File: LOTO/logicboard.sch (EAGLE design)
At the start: 31 parts, among them IC1 74ALS08N, IC2 74ALS08N, Q1 BSS92, Q2 BSS101

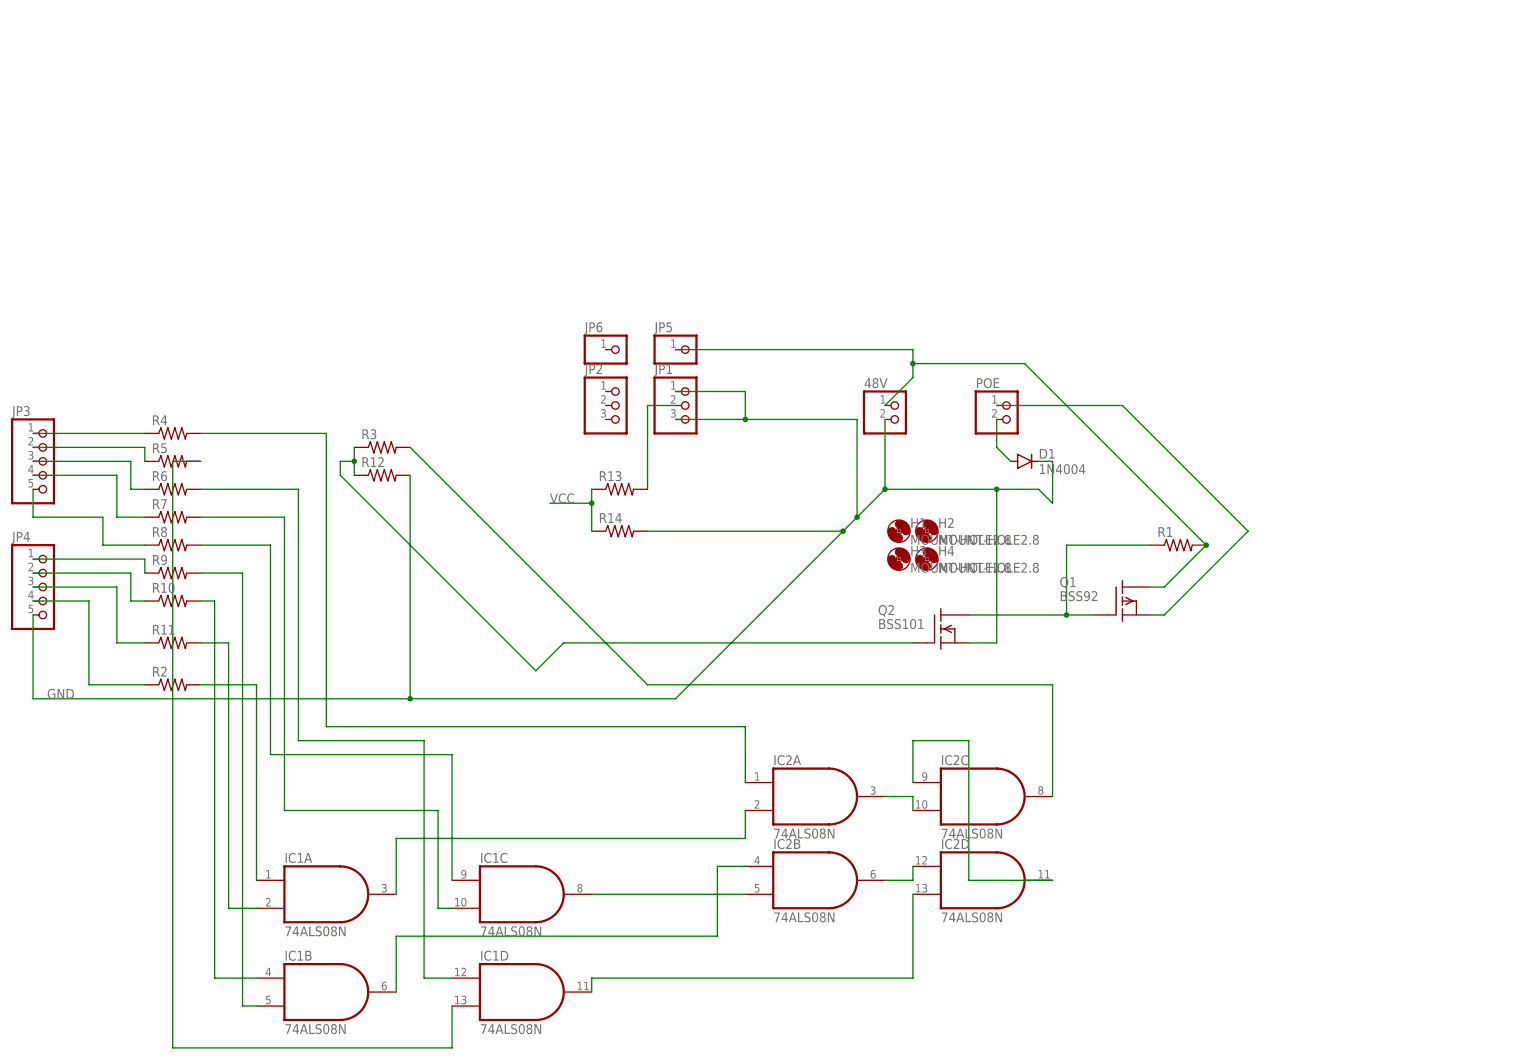
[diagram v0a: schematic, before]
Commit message: route management
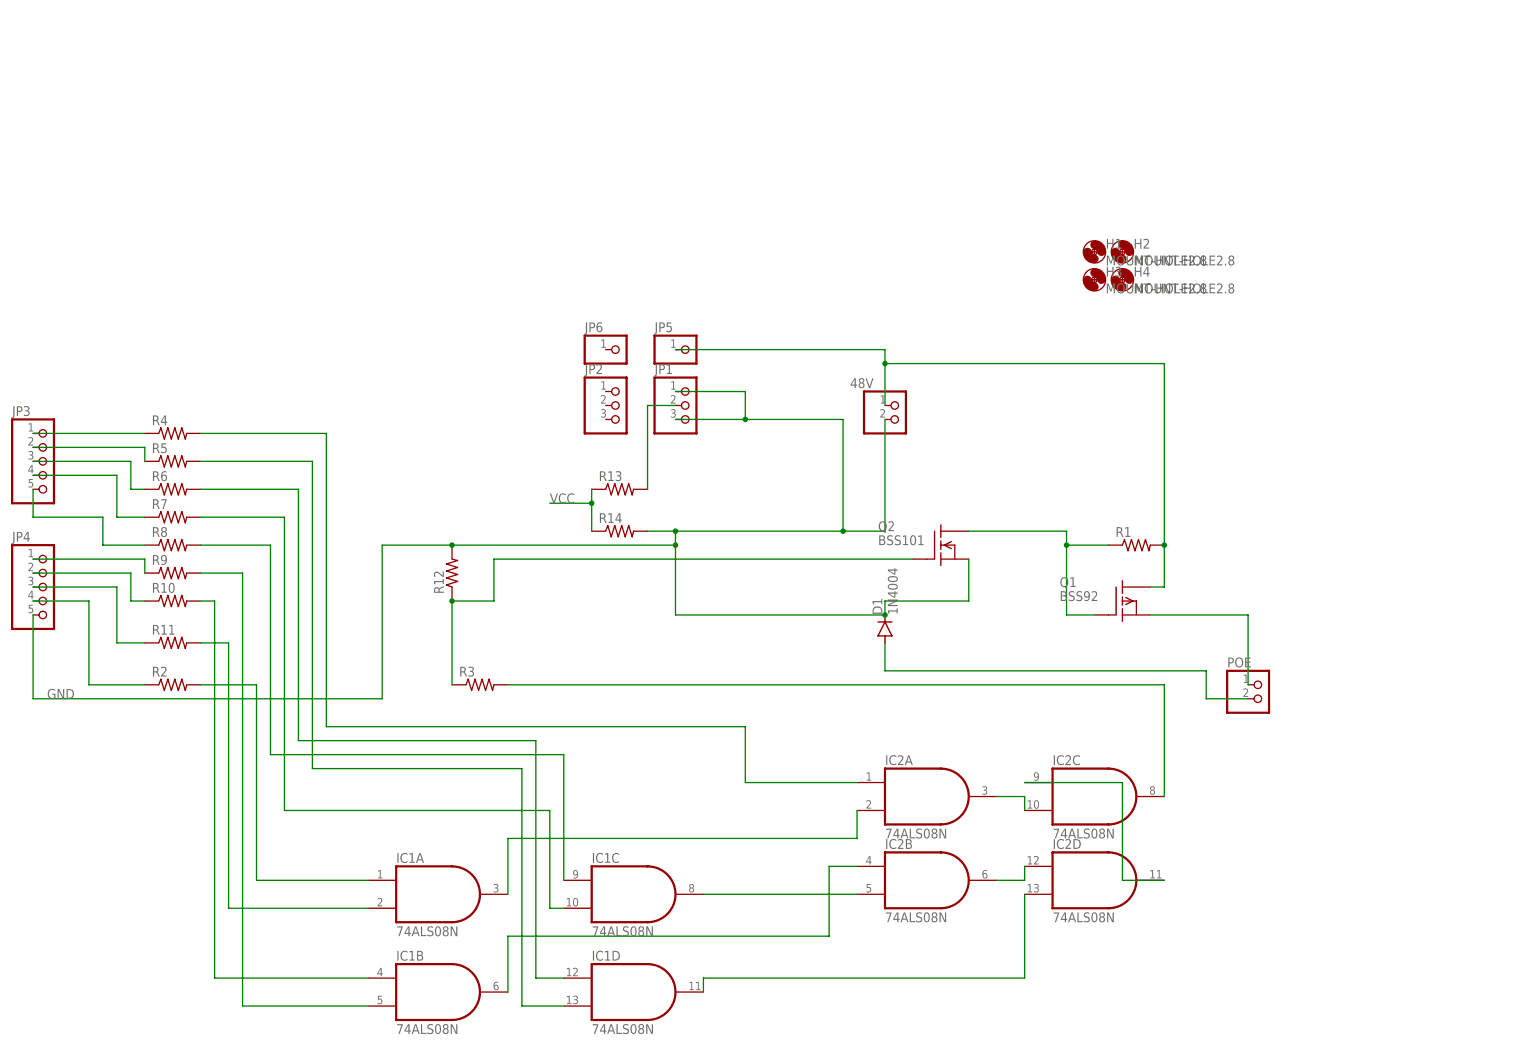
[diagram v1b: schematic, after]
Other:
- moved on the sheet: D1, H1, H2, H3, H4, IC1A, IC1B, IC1C, IC1D, IC2A, IC2B, IC2C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

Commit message: reduced AC board size, attributes, bom
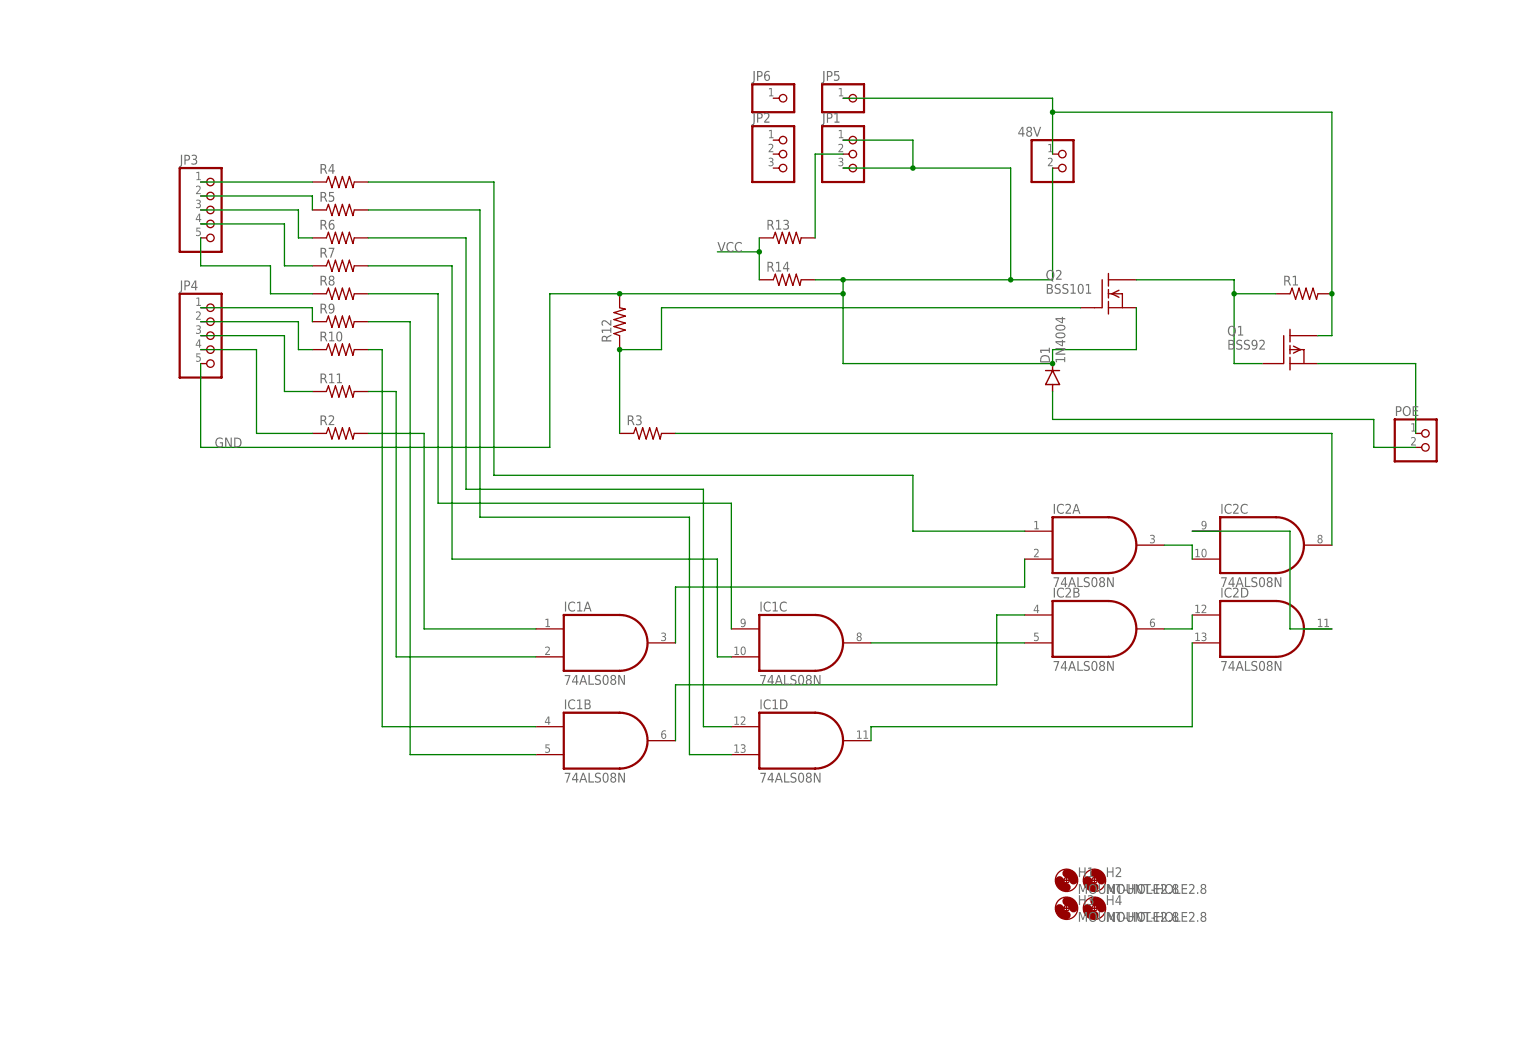
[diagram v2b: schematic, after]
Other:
- moved on the sheet: 48V, D1, H1, H2, H3, H4, IC1A, IC1B, IC1C, IC1D, IC2A, IC2B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

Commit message: added attributes to loto
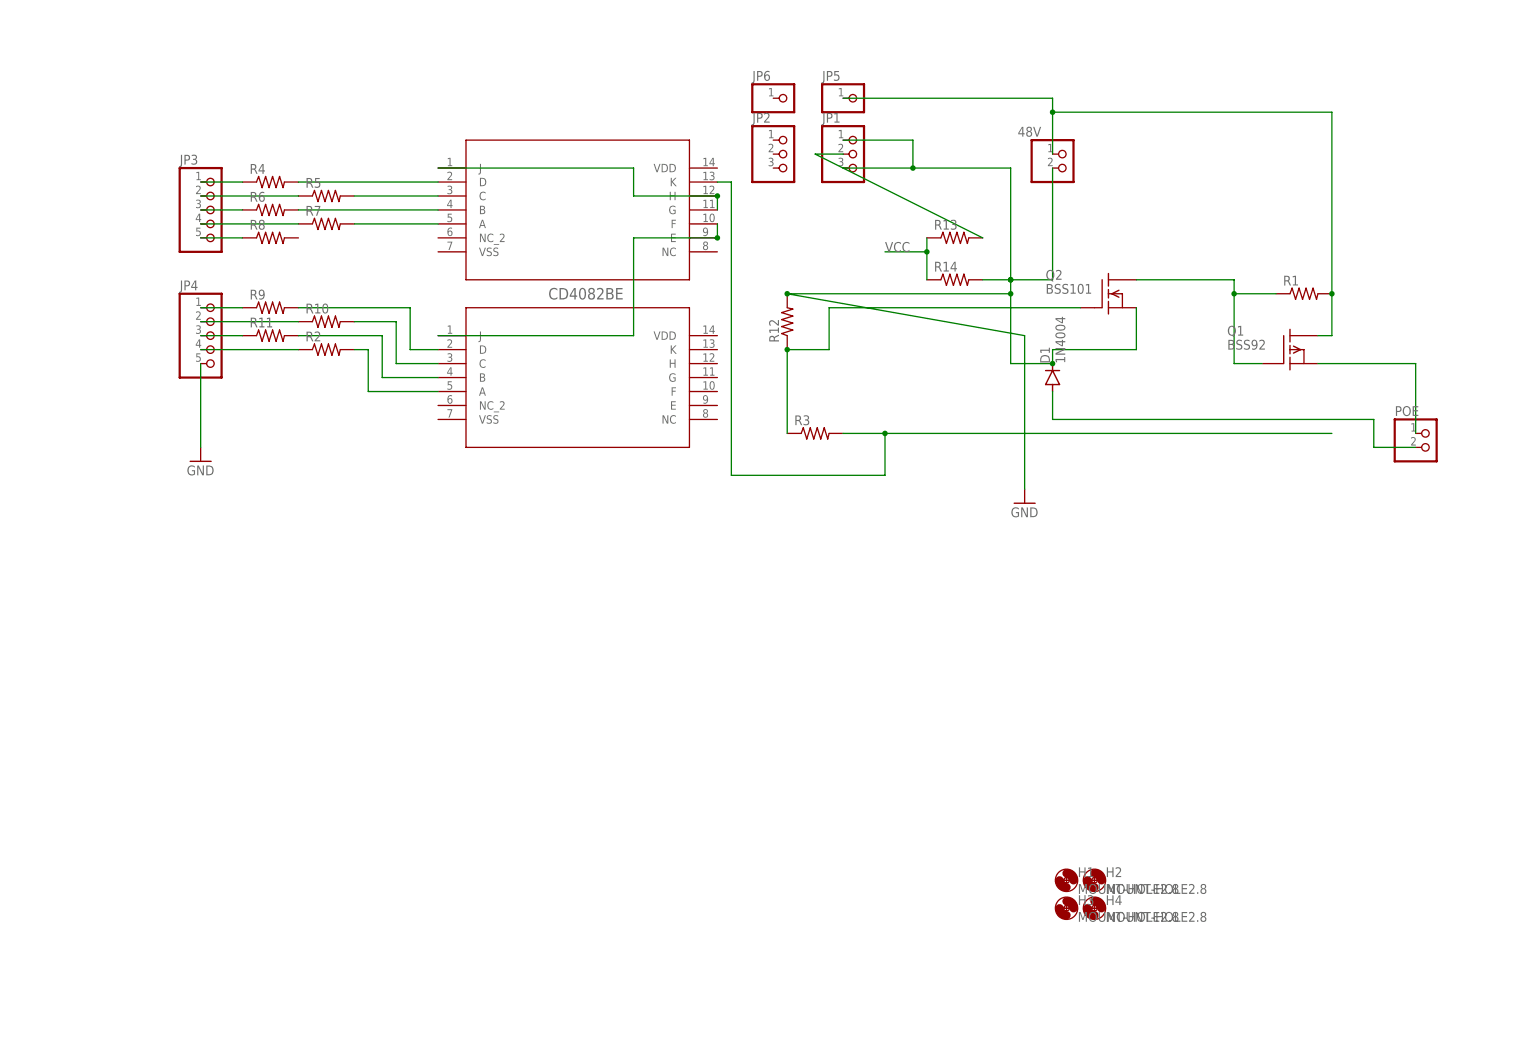
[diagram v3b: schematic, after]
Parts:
- removed IC1, IC2: 74ALS08N, 74xx-us:74ALS08N
- added U1, U2: CD4082BE, CD4082BE:CD4082BE
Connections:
- removed net N$21: IC1B.O, IC2B.I0
- removed net N$22: IC1C.O, IC2B.I1
- removed net N$23: IC1D.O, IC2D.I1
- removed net N$24: IC2B.O, IC2D.I0
- removed net N$25: IC2A.O, IC2C.I1
- removed net N$26: IC2C.I0, IC2D.O
- removed net N$33: IC1C.I1, R7.2
- new net N$16: R9.2, U2.D
- net N$11: now also R4.2, U1.D; no longer IC1A.I0, R2.2
- net N$12: now also R5.2, U1.C; no longer IC1A.I1, R11.2
- net N$13: now also R6.2, U1.B; no longer IC1B.I0, R10.2
- net N$14: now also R7.2, U1.A; no longer IC1B.I1, R9.2
- net N$15: now also U1.E, U1.F, U2.J; no longer IC1C.I0, R8.2
- net N$17: now also R10.2, U2.C; no longer IC1D.I0, R6.2
- net N$18: now also R11.2, U2.B; no longer IC1D.I1, R5.2
- net N$19: now also R2.2, U2.A; no longer IC2A.I0, R4.2
- net N$20: now also U1.G, U1.H, U1.J; no longer IC1A.O, IC2A.I1
- net ON: now also U1.K; no longer IC2C.O
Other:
- moved on the sheet: R10, R11, R12, R13, R14, R2, R3, R4, R5, R6, R7, R8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

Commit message: Updated LOTO boards
Added LOTO housing outline.  Added logic for POE power and gate trigger. Added more circuit protection and power isolation.
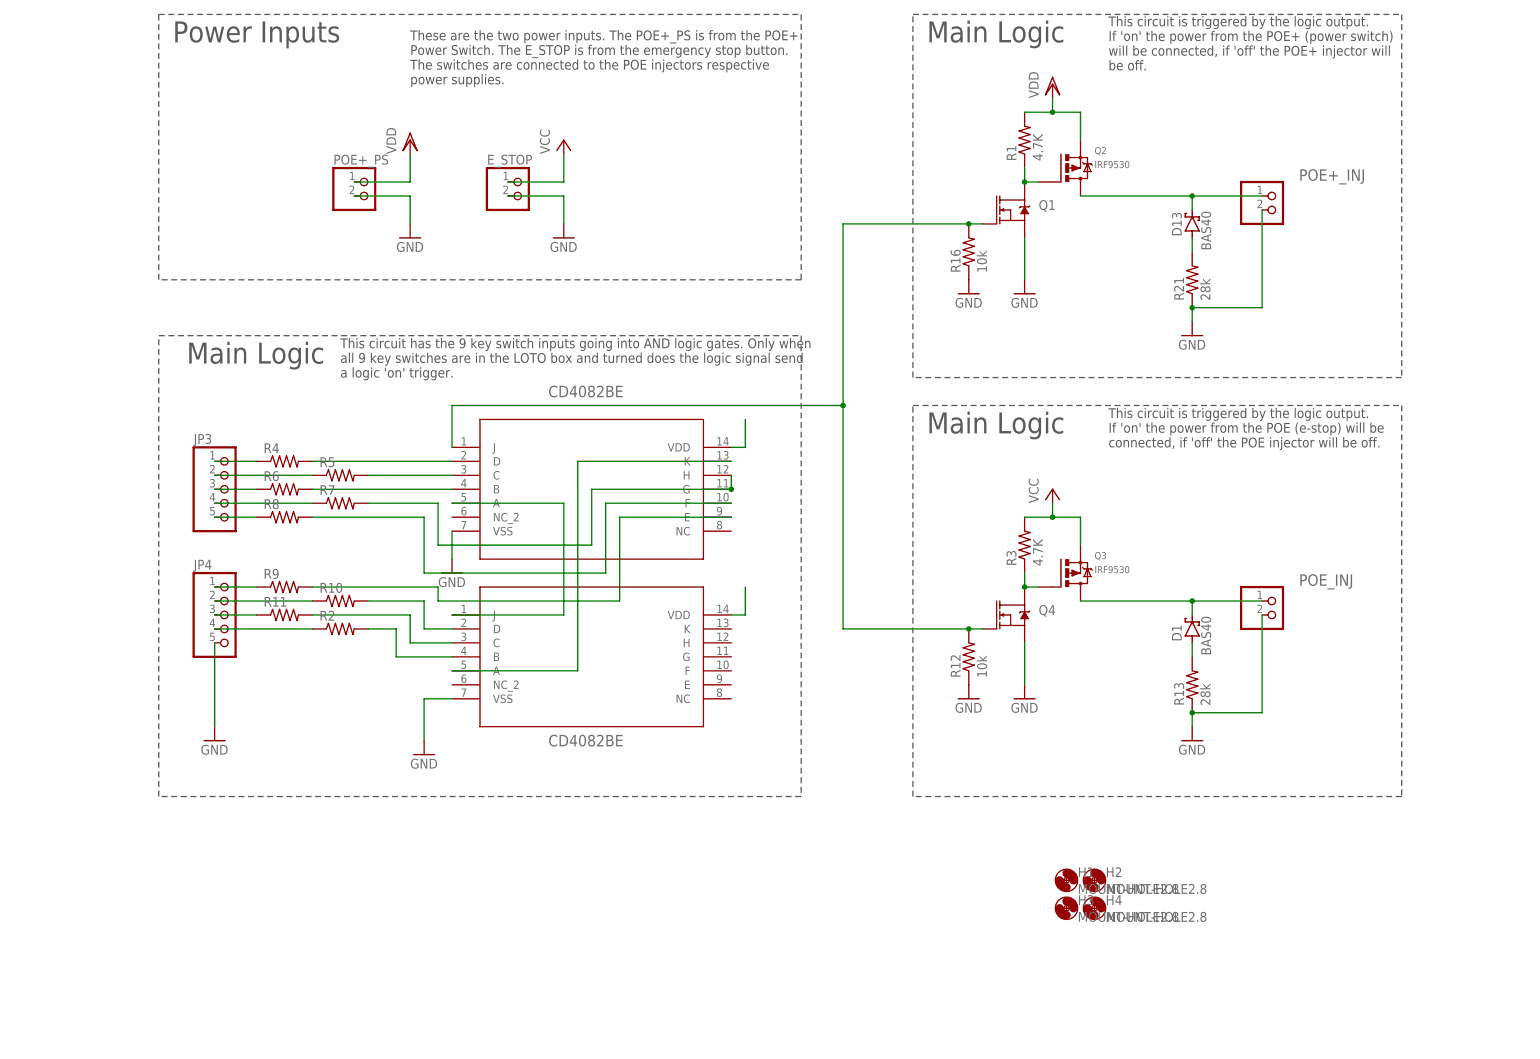
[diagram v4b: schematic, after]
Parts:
- removed 48V, POE: (no value), pinhead:PINHD-1X2
- removed JP1, JP2: (no value), pinhead:PINHD-1X3
- removed JP5, JP6: (no value), pinhead:PINHD-1X1
- removed R14: (no value), rcl:R-US_0204/5
- added D13: BAS40, diode:BAS40
- added E_STOP, POE+_INJ, POE+_PS, POE_INJ: (no value), pinhead:PINHD-1X2
- added Q3: IRF9530, transistor-power:IRF9530
- added Q4: 220mA/50V/3.5Ω, SparkFun-DiscreteSemi:MOSFET-NCH-BSS138
- added R16: 10k, oresat-rcl:R-US_0805-A-NOSILK
- added R21: 28k, oresat-rcl:R-US_0805-A-NOSILK
- D1: value 1N4004 -> BAS40; device diode:1N4004 -> diode:BAS40; DIS (none) -> Digi-Key; DPN (none) -> 1514-CMPSH1-4TRPBFREECT-ND; MFR (none) -> Central Semiconductor Corp; MPN (none) -> CMPSH1-4 TR PBFREE
- Q1: value BSS92 -> 220mA/50V/3.5Ω; device transistor-fet:BSS92 -> SparkFun-DiscreteSemi:MOSFET-NCH-BSS138; DIS (none) -> Digi-Key; DPN (none) -> 1727-1142-1-ND; MFR (none) -> Nexperia USA Inc.; MPN (none) -> BSS138P,215
- Q2: value BSS101 -> IRF9530; device transistor-fet:BSS101 -> transistor-power:IRF9530; DIS (none) -> Digi-Key; DPN (none) -> IRF9530NPBF-ND; MFR (none) -> Infineon Technologies; MPN (none) -> IRF9530NPBF
- R1, R3: value (none) -> 4.7K; device rcl:R-US_0204/5 -> oresat-rcl:R-US_0805-A-NOSILK; DIS (none) -> Digi-Key; DPN (none) -> 311-4.70KCRCT-ND; MFR (none) -> Yageo; MPN (none) -> RC0805FR-074K7L
- R12: value (none) -> 10k; device rcl:R-US_0204/5 -> oresat-rcl:R-US_0805-A-NOSILK; DIS (none) -> Digi-Key; DPN (none) -> 311-10.0KCRCT-ND; MFR (none) -> Yageo; MPN (none) -> RC0805FR-0710KL
- R13: value (none) -> 28k; device rcl:R-US_0204/5 -> oresat-rcl:R-US_0805-A-NOSILK; DIS (none) -> Digi-Key; DPN (none) -> RMCF0805FT28K0CT-ND; MFR (none) -> Stackpole Electronics Inc; MPN (none) -> RMCF0805FT28K0
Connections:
- removed net N$27: D1.A, POE.2
- removed net N$28: 48V.1, JP5.1, Q1.D, R1.2
- removed net N$29: Q2.G, R12.1, R3.1
- removed net N$30: Q1.G, Q2.D, R1.1
- removed net N$32: JP1.2, R13.2
- new net N$21: U1.K, U2.A
- new net N$22: D1.A, R13.2
- new net N$23: Q3.G, Q4.D, R3.1
- new net N$24: U2.VDD
- new net N$25: U1.VDD
- new net N$54: D13.A, R21.2
- new net SOL_GPIO_1: D1.C, POE_INJ.1, Q3.D
- new net SOL_GPIO_10: D13.C, POE+_INJ.1, Q2.D
- new net VDD: POE+_PS.1, Q2.S, R1.2
- net GND: now also E_STOP.2, POE+_INJ.2, POE+_PS.2, POE_INJ.2, Q1.S, Q4.S, R12.1, R13.1, R16.1, R21.1, U1.VSS, U2.VSS; no longer 48V.2, D1.C, JP1.1, JP1.3, Q2.S, R12.2, R14.2
- net N$10: now also Q1.D, Q2.G, R1.1; no longer POE.1, Q1.S
- net N$14: now also U1.G, U1.H; no longer U1.A
- net N$15: now also R8.2; no longer U1.E, U2.J
- net N$16: now also U1.E; no longer U2.D
- net N$17: now also U2.D; no longer U2.C
- net N$18: now also U2.C; no longer U2.B
- net N$19: now also U2.B; no longer U2.A
- net N$20: now also U1.A, U2.J; no longer U1.G, U1.H, U1.J
- net ON: now also Q1.G, Q4.G, R12.2, R16.2, U1.J; no longer R3.2, U1.K
- net VCC: now also E_STOP.1, Q3.S, R3.2; no longer R13.1, R14.1
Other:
- note added: "Main Logic"
- note added: "Power Inputs"
- note added: "These are the two power inputs. The POE+_PS is from the POE+ Power Switch. The E_STOP is from the emergency stop button. The switches are connected to the POE injectors respective power supplies."
- note added: "This circuit has the 9 key switch inputs going into AND logic gates. Only when all 9 key switches are in the LOTO box and turned does the logic signal send a logic 'on' trigger."
- note added: "This circuit is triggered by the logic output. If 'on' the power from the POE (e-stop) will be connected, if 'off' the POE injector will be off."
- note added: "This circuit is triggered by the logic output. If 'on' the power from the POE+ (power switch) will be connected, if 'off' the POE+ injector will be off."
- moved on the sheet: JP3, JP4, R10, R11, R2, R4, R5, R6, R7, R8, R9
